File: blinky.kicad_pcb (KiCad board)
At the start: 2 copper layers, 34 x 30.5 mm, 7 parts, among them U1 7555

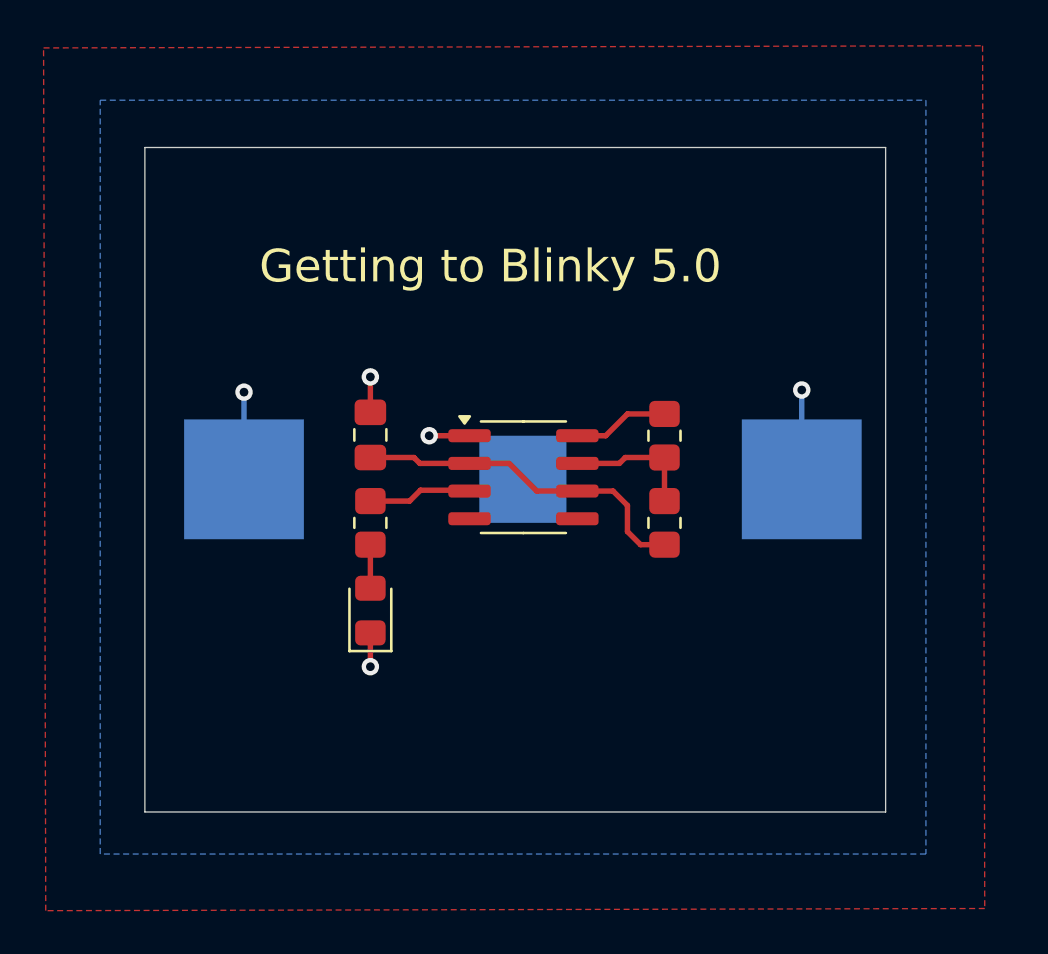
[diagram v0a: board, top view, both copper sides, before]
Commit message: Add fabrication files
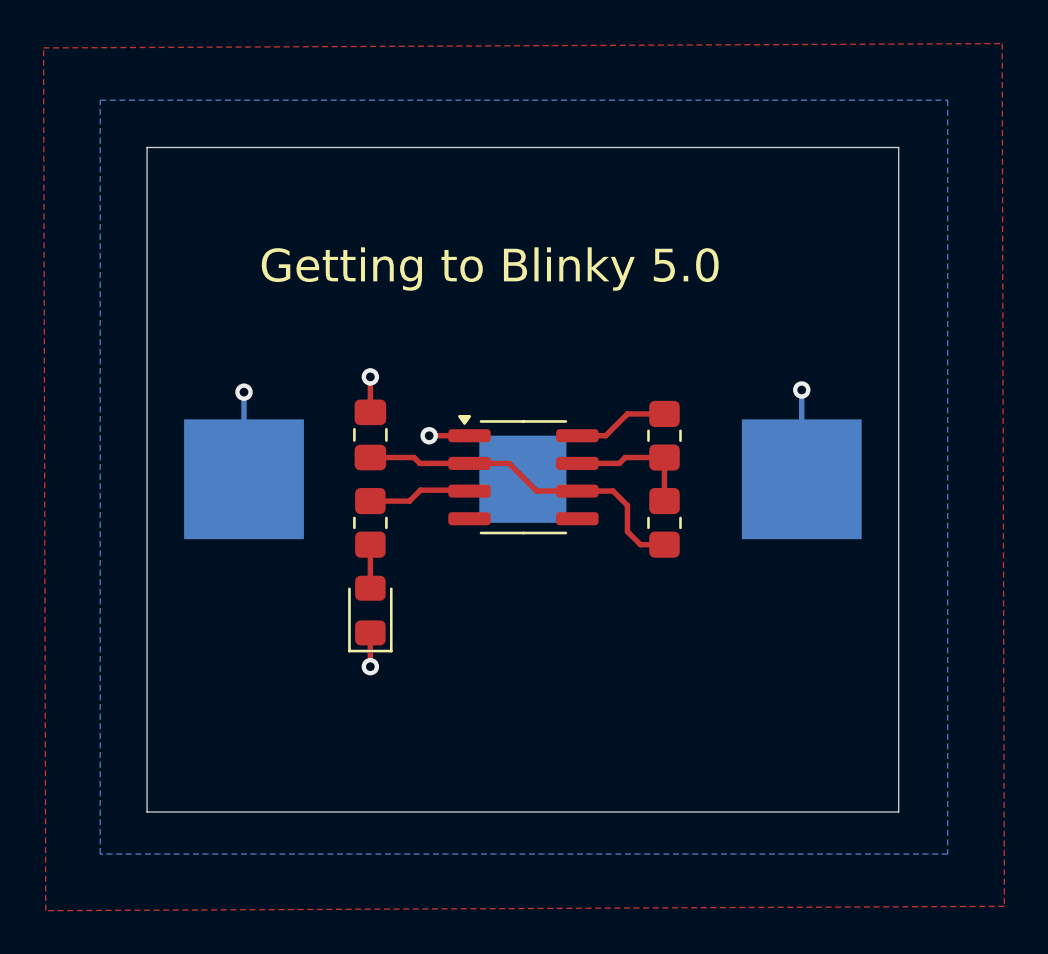
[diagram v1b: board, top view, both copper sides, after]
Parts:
- C1: value 1U -> 1uf
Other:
- board size 34 x 30.5 mm -> 34.5 x 30.5 mm
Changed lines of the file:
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@@
 			(outputformat 1)
 			(mirror no)
-			(drillshape 1)
+			(drillshape 0)
 			(scaleselection 1)
-			(outputdirectory "")
+			(outputdirectory "Fabrication/Gerbers/")
 		)
 	)
@@
 			)
 		)
-		(property "Value" "1U"
+		(property "Value" "1uf"
 			(at 0 1.68 90)
 			(layer "F.Fab")
@@
 	)
 	(gr_rect
-		(start 87.85 43.97)
-		(end 121.85 74.47)
+		(start 87.95 43.97)
+		(end 122.45 74.47)
 		(stroke
 			(width 0.05)
@@
 		(polygon
 			(pts
-				(xy 126.3 39.3) (xy 126.4 78.9) (xy 83.3 79) (xy 83.2 39.4)
+				(xy 127.2 39.2) (xy 127.3 78.8) (xy 83.3 79) (xy 83.2 39.4)
 			)
 		)
@@
 		(polygon
 			(pts
-				(xy 123.7 41.8) (xy 123.7 76.4) (xy 85.8 76.4) (xy 85.8 41.8)
-			)
-		)
+				(xy 124.7 41.8) (xy 124.7 76.4) (xy 85.8 76.4) (xy 85.8 41.8)
+			)
+		)
